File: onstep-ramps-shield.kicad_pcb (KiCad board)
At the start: 2 copper layers, 120.6 x 67.3 mm, 30 parts

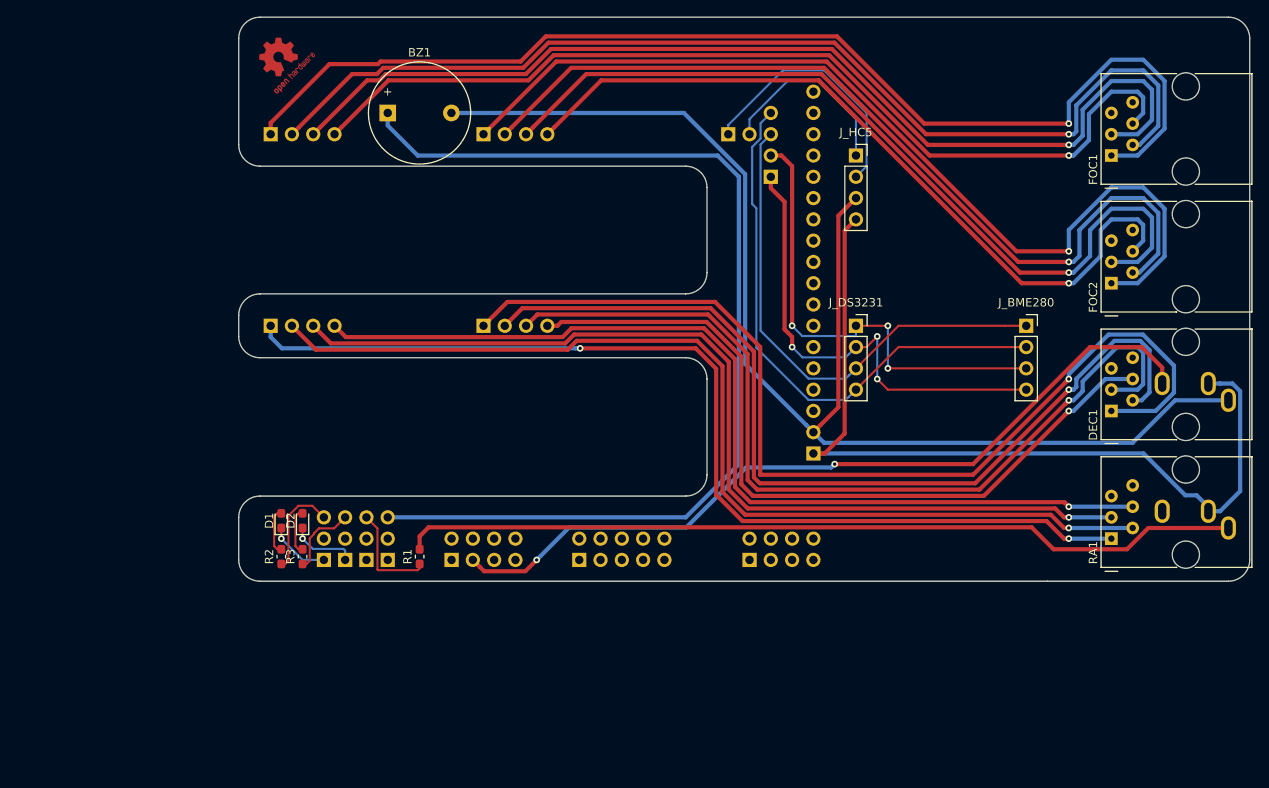
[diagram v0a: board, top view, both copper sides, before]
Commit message: Measured distances
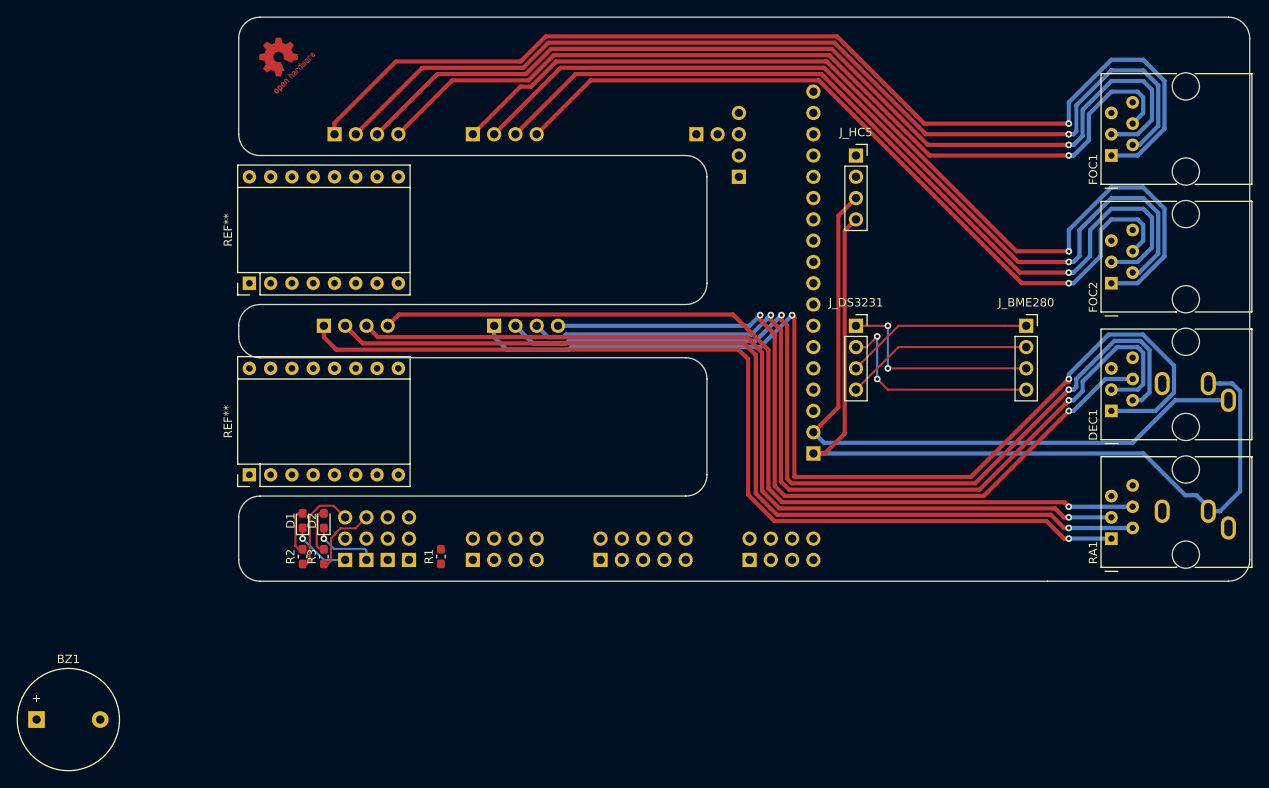
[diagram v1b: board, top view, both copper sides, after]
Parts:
- added REF**: Pololu_Breakout-16_15.2x20.3mm, Module:Pololu_Breakout-16_15.2x20.3mm, F.Cu at (83.8, 82.5)
- added REF**: Pololu_Breakout-16_15.2x20.3mm, Module:Pololu_Breakout-16_15.2x20.3mm, F.Cu at (83.8, 105.4)
- moved BZ1 83.6 mm to (58.4, 134.6)
- moved J_FOC1 7.62 mm to (94.0, 64.8)
- moved J_RA1 6.35 mm to (92.7, 87.6)
- moved J_I2C1 3.81 mm to (142.2, 69.8)
- moved J_SER1 3.81 mm to (137.2, 64.8)
- moved D1 2.54 mm to (90.2, 110.9)
- moved J_AUX2 2.54 mm to (125.7, 115.6)
- moved J_SERV1 2.54 mm to (95.2, 115.6)
- moved J_SERV2 2.54 mm to (97.8, 115.6)
- moved J_SERV4 2.54 mm to (102.9, 115.6)
- moved R1 2.54 mm to (106.7, 115.2)
- moved R2 2.54 mm to (90.2, 115.2)
- moved D2 2.54 mm to (92.7, 110.9)
- moved J_AUX1 2.54 mm to (110.5, 115.6)
- moved J_SERV3 2.54 mm to (100.3, 115.6)
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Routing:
- net BUZZER1: track 124.8 -> 0.00 mm
- net Net-(J_RET1-PadS): track 100.7 -> 0.00 mm
- net PEC1: track 96.8 -> 0.00 mm, vias 2 -> 0
- net GND: track 154.5 -> 82.2 mm
- net I2C_SCL: track 66.5 -> 22.4 mm
- net I2C_SDA: track 60.6 -> 22.4 mm
- net GND_I2C1: track 56.8 -> 25.4 mm, vias 3 -> 2
- net RX1: track 30.6 -> 0.00 mm
- net VCC_I2C1: track 56.5 -> 26.5 mm, vias 3 -> 2
- net TX1: track 22.6 -> 0.00 mm
- net RETICULE_LED1: track 12.5 -> 0.00 mm
- net E0_1A: track 123.6 -> 116.0 mm
- net E0_2B: track 135.7 -> 128.1 mm
- net E0_2A: track 127.0 -> 119.4 mm
- net E0_1B: track 114.3 -> 106.7 mm
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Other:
- outline, holes or cut-outs redrawn
